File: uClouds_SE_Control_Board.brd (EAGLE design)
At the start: 40 x 110.5 mm, 38 parts, among them J1 JACK-THONKICONN, J10 JACK-THONKICONN, J11 JACK-THONKICONN, J12 JACK-THONKICONN, J2 JACK-THONKICONN, J3 JACK-THONKICONN, J4 JACK-THONKICONN, J5 JACK-THONKICONN, J6 JACK-THONKICONN, J7 JACK-THONKICONN, J8 JACK-THONKICONN, J9 JACK-THONKICONN, P1 10k, P2 10k, P3 A50k, P4 10k, P5 10k, P6 10k, P7 10k

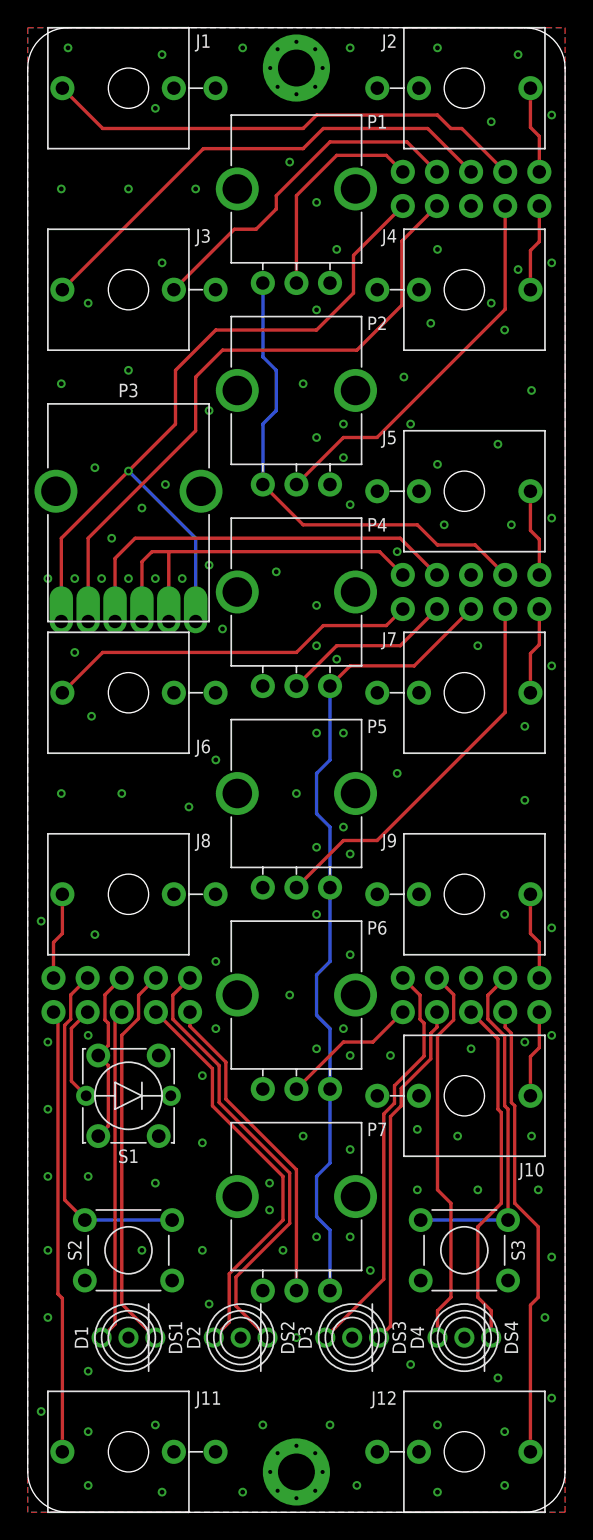
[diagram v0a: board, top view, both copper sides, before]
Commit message: Cleanup and silkscreen artwork updates
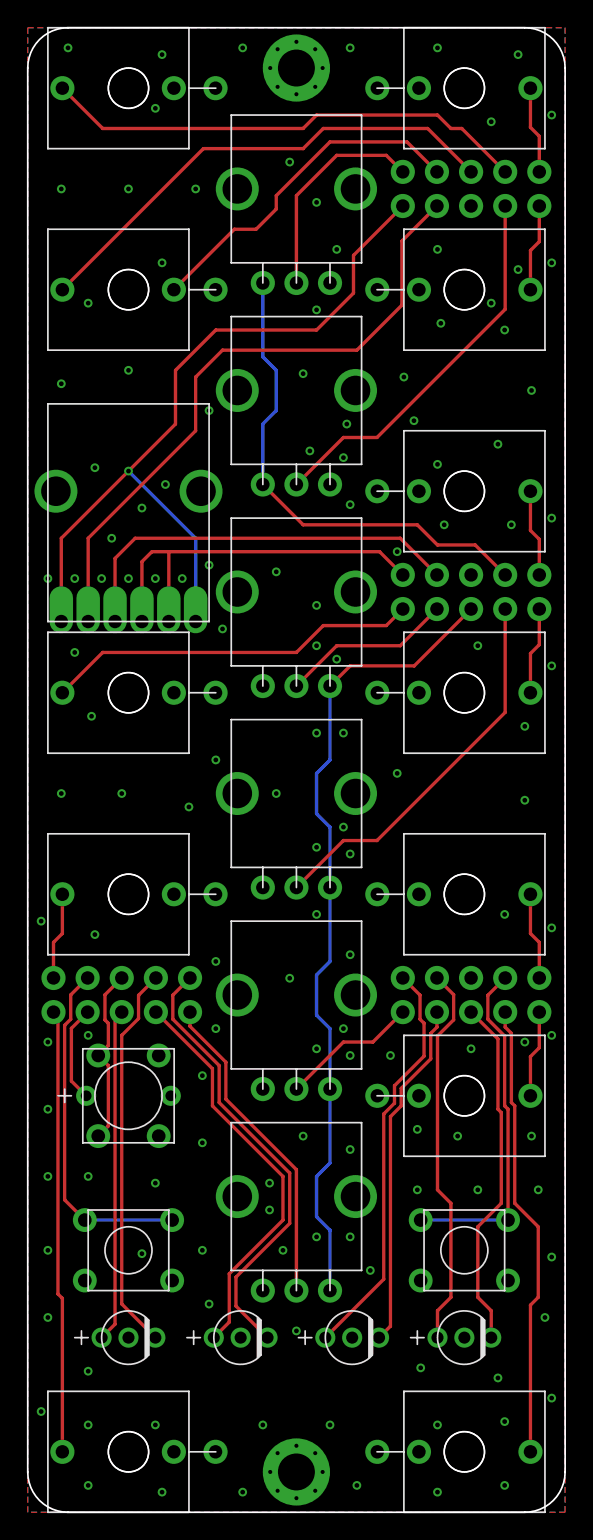
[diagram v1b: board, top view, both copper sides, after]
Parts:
- removed U$1: (no value), uClouds_SE_Library:MARKING-CC-LOGO
- removed U$2: (no value), uClouds_SE_Library:MARKING-OSH-LOGO-5MM
- H1, H2, H3, H4: device uClouds_SE_Library:PTH-0.1-2X5 -> uClouds_SE_Library:PTH-0.1-2X5-MALE
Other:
- board text added: "2019-12-18"
- board text removed: "2019-12-09"
- board text removed: "BY-SA 4.0"
- board text removed: "Board derived from work by"
- board text removed: "CC BY-SA 4.0"
- board text removed: "Control Board"
- board text removed: "open source hardware"
- board text removed: "tall-dog.com"
- board text removed: "µClouds SE"
- board text removed: "Émilie Gillet of Mutable Instruments"
